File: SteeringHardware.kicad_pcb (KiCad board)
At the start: 2 copper layers, 87 x 55.9 mm, 74 parts, among them J10 Output, J11 Input, J12 Output, J13 Input, J14 Input, J15 Output, J16 Input, J17 Output, J18 Output, J19 Input, J2 USB_B_Micro, J20 Input, J3 Main Connector, J301 Conn_ARM_JTAG_SWD_10, J4 Output, J5 Input, J6 Input, J7 Output, J8 Input, J9 Input, Q1 AO3400A, Q101 MMBT2222, Q2 AO3400A, Q3 AO3400A, Q4 AO3400A, Q5 AO3400A, Q6 AO3400A, Q7 AO3400A, U101 DISP_LCD_1.28IN_240x320_50Pin, U102 AMS1117-5.0, U201 TPS5430DDA, U3 TPS2113, U301 STM32F072RBTx, U4 TCAN1042xV

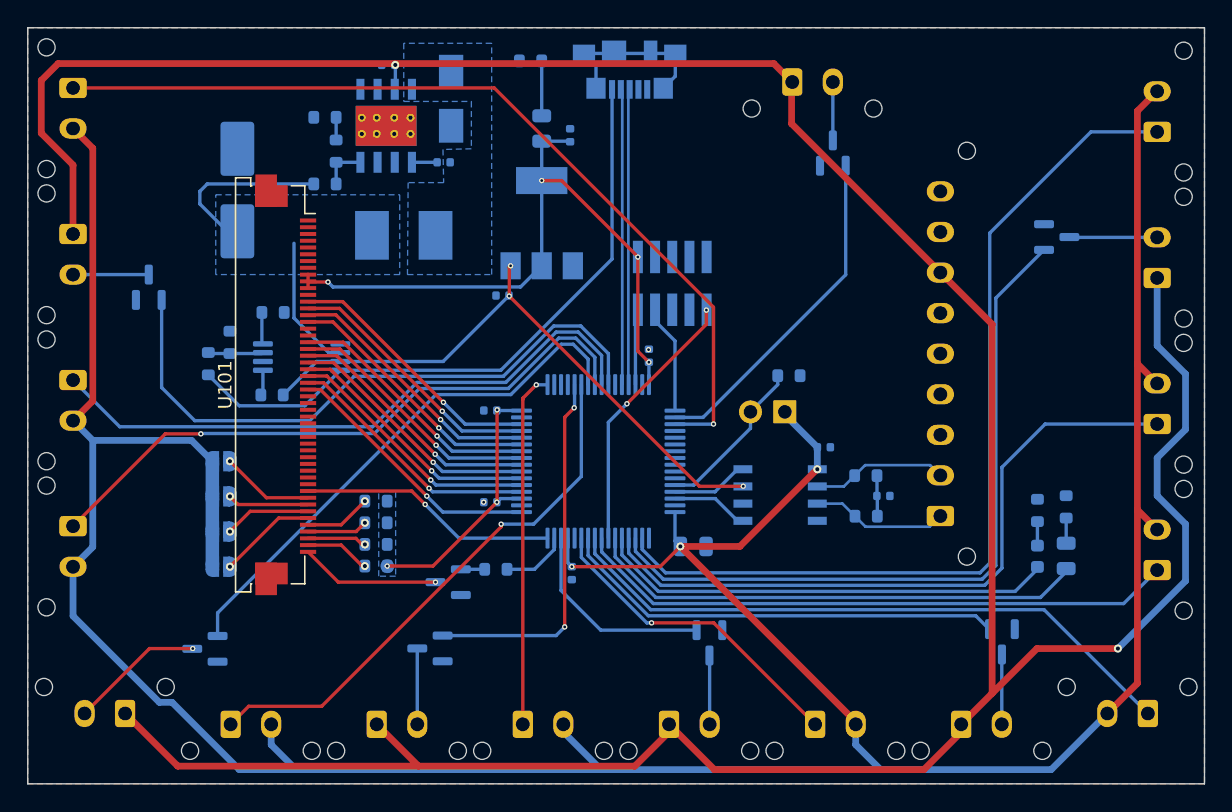
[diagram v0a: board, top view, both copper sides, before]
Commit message: Current board
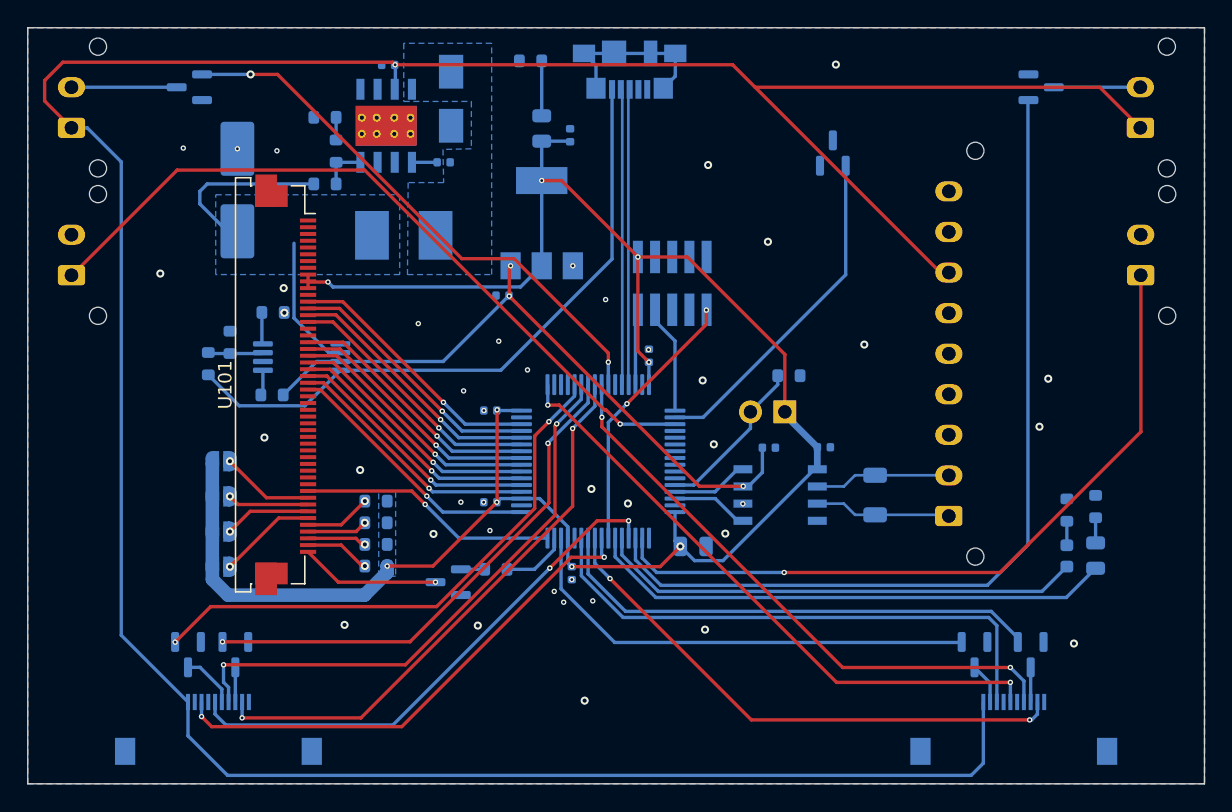
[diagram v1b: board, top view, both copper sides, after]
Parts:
- removed J10, J12, J15, J17, J18, J4, J7: Output, Connector_Molex:Molex_Micro-Fit_3.0_43650-0215_1x02_P3.00mm_Vertical
- removed J11, J13, J14, J16, J19, J20, J5, J6, J8, J9: Input, Connector_Molex:Molex_Micro-Fit_3.0_43650-0215_1x02_P3.00mm_Vertical
- removed R12: 60, Resistor_SMD:R_0603_1608Metric
- added J101: Conn1, JohnLib:Connector_FPC_Molex_2004850410, B.Cu at (145.9, 114.3)
- added J102: Conn2, JohnLib:Connector_FPC_Molex_2004850410, B.Cu at (204.7, 114.3)
- added J103: RT_LED, Connector_Molex:Molex_Micro-Fit_3.0_43650-0215_1x02_P3.00mm_Vertical, B.Cu at (214.1, 71.9)
- added J104: RT_BTN, Connector_Molex:Molex_Micro-Fit_3.0_43650-0215_1x02_P3.00mm_Vertical, B.Cu at (214.1, 82.8)
- added J105: LT_LED, Connector_Molex:Molex_Micro-Fit_3.0_43650-0215_1x02_P3.00mm_Vertical, B.Cu at (135.0, 71.9)
- added J106: LT_BTN, Connector_Molex:Molex_Micro-Fit_3.0_43650-0215_1x02_P3.00mm_Vertical, B.Cu at (135.0, 82.8)
- R11: value 60 -> 120; footprint Resistor_SMD:R_0603_1608Metric -> Resistor_SMD:R_1206_3216Metric
- moved Q6 19.6 mm to (201.8, 110.8)
- moved Q5 17.9 mm to (143.7, 110.8), turned to -90 degrees
- moved Q1 15.1 mm to (143.8, 68.9), turned to 180 degrees
- moved Q2 11.1 mm to (206.7, 68.9)
- moved C2 9.19 mm to (186.6, 95.5)
- moved Q3 2.33 mm to (205.9, 110.8)
- moved Q4 2.29 mm to (147.2, 110.8), turned to -90 degrees
- moved D1 2.18 mm to (210.8, 103.5)
- moved D2 2.18 mm to (208.6, 103.5)
- moved R1 2.18 mm to (210.8, 99.9)
- moved R2 2.18 mm to (208.6, 100.2)
- moved R11 1.59 mm to (194.4, 99.0), turned to -90 degrees
- moved J3 0.62 mm to (199.9, 100.6)
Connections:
- C2 pad 1: Net-(C2-Pad1) -> +5V
- Q1 pad 1: /LT_LED -> /LT_LED_EN
- Q1 pad 3: Net-(J4-Pad2) -> /LT_LED
- Q2 pad 1: /RT_LED -> /RT_LED_EN
- Q2 pad 3: Net-(J7-Pad2) -> /RT_LED
- Q3 pad 1: /Cruise_ON -> /Cruise_ON_EN
- Q3 pad 3: Net-(J10-Pad2) -> /Cruise_ON
- Q4 pad 1: /ECO_ON -> /ECO_ON_EN
- Q4 pad 3: Net-(J12-Pad2) -> /ECO_ON
- Q5 pad 1: /Headlights_ON -> /Headlights_ON_EN
- Q5 pad 3: Net-(J15-Pad2) -> /Headlights_ON
- Q6 pad 1: /Rev_ON -> /Rev_ON_EN
- Q6 pad 3: Net-(J17-Pad2) -> /Rev_ON
- Q7 pad 1: /BPS_Fault -> /BPS_Fault_EN
- Q7 pad 3: Net-(J18-Pad2) -> /BPS_Fault
- R11 pad 2: Net-(C2-Pad1) -> /CAN+
- U301 pad 10: /Cruise_ON -> /Cruise_ON_EN
- U301 pad 14: /Rev_ON -> /Rev_ON_EN
- U301 pad 3: /RT_LED -> /RT_LED_EN
- U301 pad 37: /Headlights_ON -> /Headlights_ON_EN
- U301 pad 39: /ECO_ON -> /ECO_ON_EN
- U301 pad 42: /LT_LED -> /LT_LED_EN
- U301 pad 50: /BPS_Fault -> /BPS_Fault_EN
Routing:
- net +3V3: track 322.2 -> 148.8 mm, vias 10 -> 9
- net /RT_LED_EN: track 0.00 -> 65.5 mm
- net /RT_LED: track 53.7 -> 6.40 mm
- net /Headlights_ON_EN: track 0.00 -> 41.1 mm, vias 0 -> 2
- net /LT_LED_EN: track 0.00 -> 40.9 mm, vias 0 -> 2
- net /LT_LED: track 46.6 -> 7.78 mm
- net /ECO_ON_EN: track 0.00 -> 38.4 mm, vias 0 -> 2
- net /ECO_ON: track 39.7 -> 2.56 mm
- net /Cruise_ON_EN: track 0.00 -> 36.4 mm
- net /Rev_ON_EN: track 0.00 -> 35.0 mm
- net /Cruise_ON: track 33.2 -> 2.56 mm
- net /BPS_Fault_EN: track 0.00 -> 25.0 mm
- net /BPS_Fault: track 25.0 -> 0.00 mm
- net /Headlights_ON: track 27.5 -> 4.12 mm, vias 2 -> 0
- net /HAZ: track 26.3 -> 45.6 mm, vias 1 -> 2
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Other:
- board text removed: "+"
- board text removed: "C+_B"
- board text removed: "C-_B"
- board text removed: "CR_L"
- board text removed: "Cr_B"
- board text removed: "E_B"
- board text removed: "Eco_L"
- board text removed: "HL_B"
- board text removed: "HL_L"
- board text removed: "Haz_B"
- board text removed: "Hrn_B"
- board text removed: "Lt_B"
- board text removed: "Lt_L"
- board text removed: "RT_B"
- board text removed: "RT_L"
- board text removed: "R_B"
- board text removed: "R_L"
- board text removed: "S"
